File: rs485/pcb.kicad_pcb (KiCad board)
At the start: 4 copper layers, 66.8 x 22 mm, 33 parts, among them J1 RJ45_LED, J2 CONN_02X06_Odd_Even, U1 LDO, U2 sp485, U3 sp485, U4 sp485

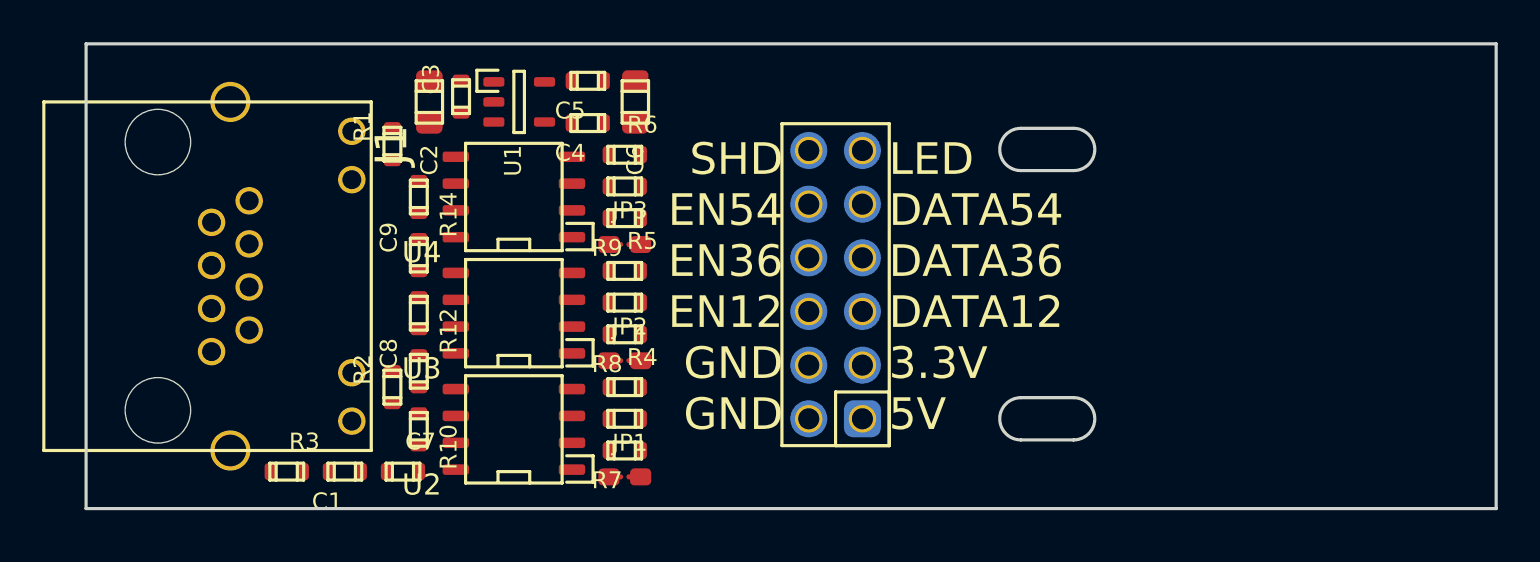
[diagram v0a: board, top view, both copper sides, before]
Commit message: hw
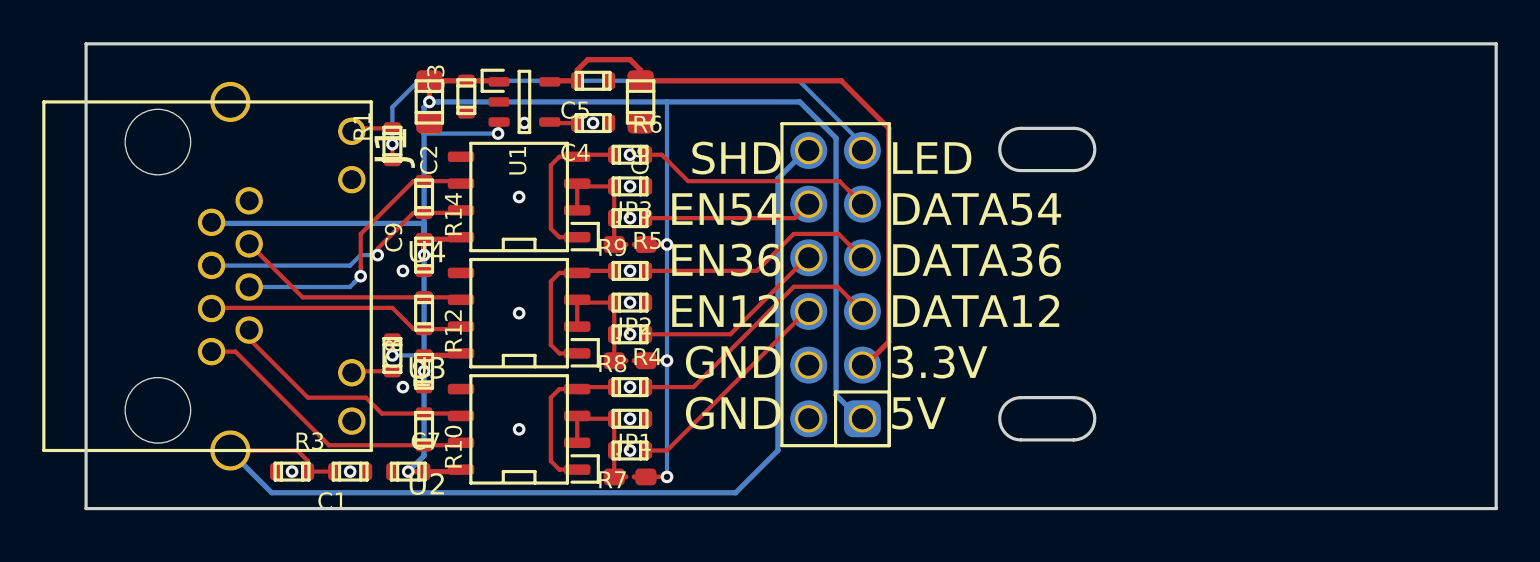
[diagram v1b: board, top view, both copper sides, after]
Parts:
- moved R2 1.50 mm to (105.2, 62.2), turned to 90 degrees
- moved C1 0.25 mm to (103.2, 67.8)
- moved C3 0.25 mm to (108.8, 50.0)
- moved C4 0.25 mm to (114.8, 51.2)
- moved C5 0.25 mm to (114.8, 49.2)
- moved C6 0.25 mm to (117.0, 50.2)
- moved C7 0.25 mm to (106.0, 67.8)
- moved C8 0.25 mm to (106.8, 63.0)
- moved C9 0.25 mm to (106.8, 57.5)
- moved JP1 0.25 mm to (116.5, 68.0)
- moved JP2 0.25 mm to (116.5, 62.5)
- moved JP3 0.25 mm to (116.5, 57.0)
- moved R10 0.25 mm to (106.8, 65.8)
- moved R11 0.25 mm to (116.5, 65.2)
- moved R12 0.25 mm to (106.8, 60.2)
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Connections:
- R2 pad 2: +3V3 -> +5V
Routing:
- net +5V: track 0.00 -> 102.3 mm, vias 0 -> 9
- net GNDS: track 0.00 -> 48.1 mm
- net +3V3: track 0.00 -> 30.2 mm
- net LED: track 0.00 -> 26.8 mm, vias 0 -> 1
- net 1: track 0.00 -> 13.7 mm
- net 4: track 0.00 -> 13.3 mm, vias 0 -> 1
- net 5: track 0.00 -> 13.1 mm, vias 0 -> 1
- net Net-(J2-Pad5): track 0.00 -> 12.7 mm
- net 3: track 0.00 -> 12.3 mm
- net 2: track 0.00 -> 12.0 mm
- net Net-(J2-Pad7): track 0.00 -> 11.4 mm
- net Net-(J2-Pad9): track 0.00 -> 11.2 mm
- net 6: track 0.00 -> 11.1 mm
- net Net-(J2-Pad6): track 0.00 -> 10.4 mm
- net Net-(J2-Pad8): track 0.00 -> 9.21 mm
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- added copper zone on B.Cu, net GND
